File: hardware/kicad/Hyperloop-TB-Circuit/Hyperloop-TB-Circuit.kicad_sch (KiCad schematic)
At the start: 12 parts, among them J1 Conn_01x02, J2 Conn_01x02, Q1 IRLZ44N

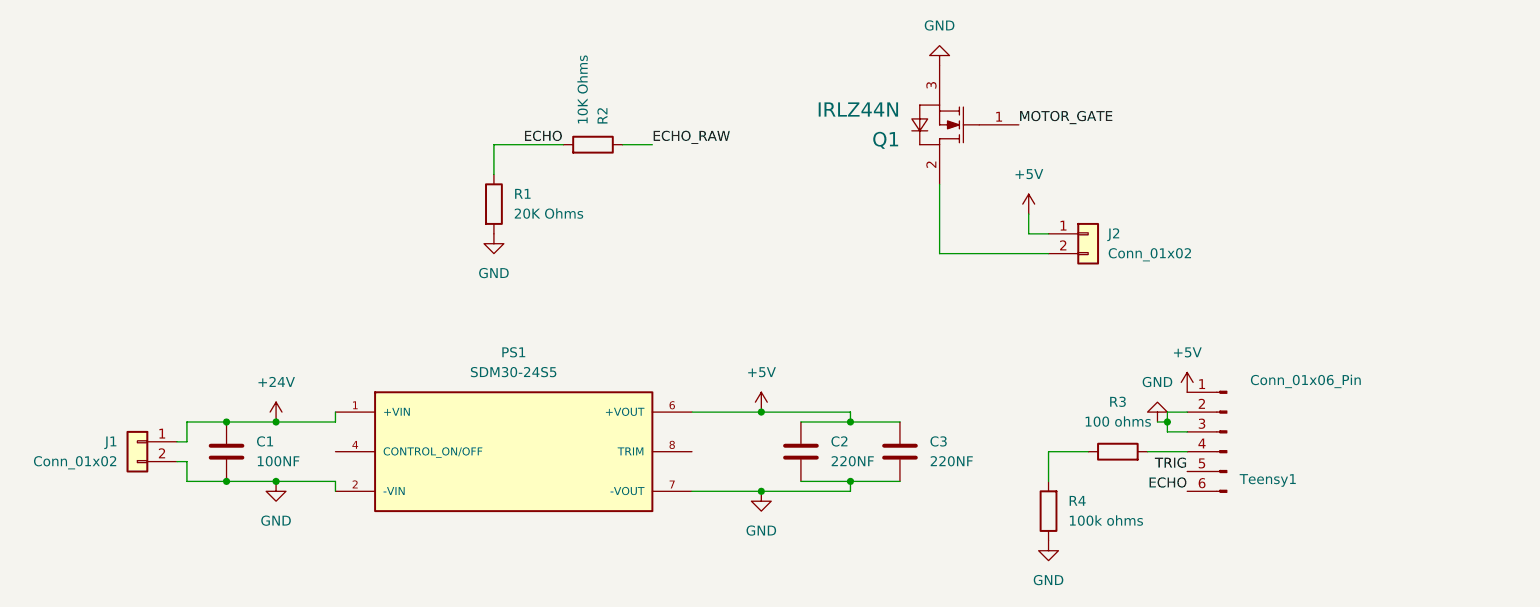
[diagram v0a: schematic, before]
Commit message: updated schematic and pcb
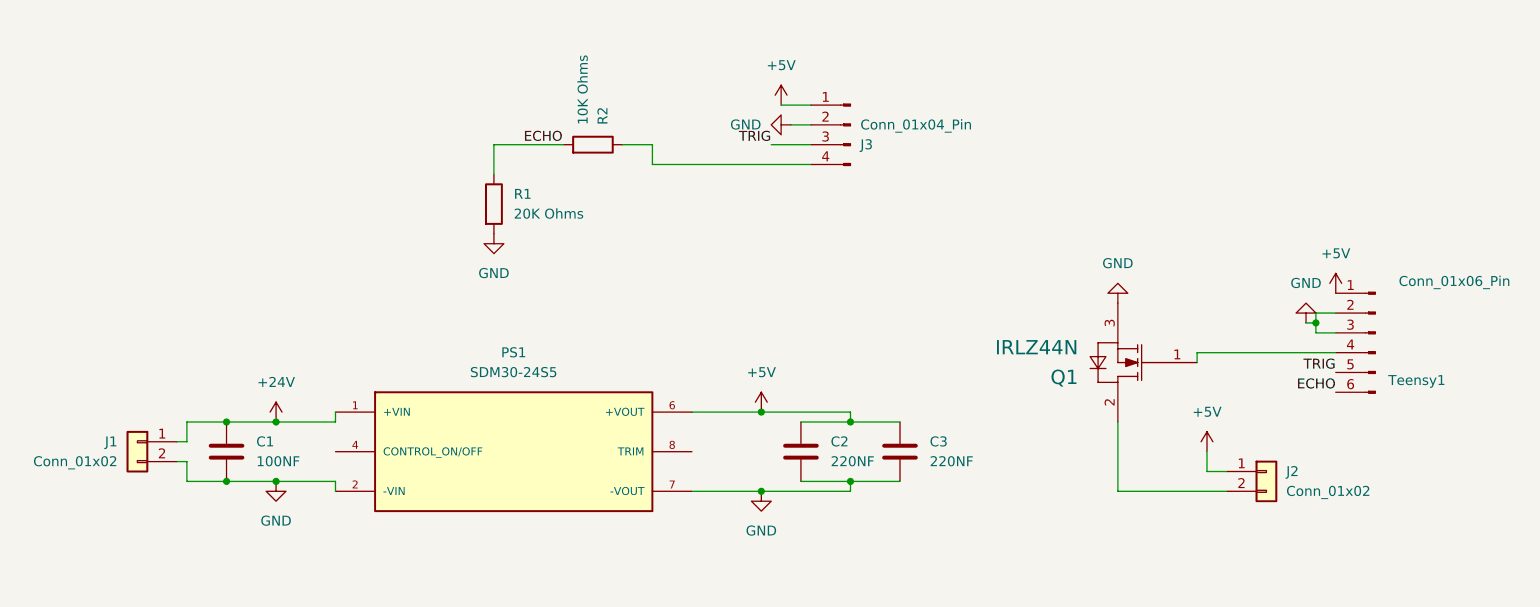
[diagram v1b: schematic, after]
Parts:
- removed R3: 100 ohms, Resistor_THT:R_Axial_DIN0204_L3.6mm_D1.6mm_P7.62mm_Horizontal, symbol Device:R
- removed R4: 100k ohms, Resistor_THT:R_Axial_DIN0204_L3.6mm_D1.6mm_P7.62mm_Horizontal, symbol Device:R
- added J3: Conn_01x04_Pin, Connector_Samtec_HPM_THT:Samtec_HPM-04-01-x-S_Straight_1x04_Pitch5.08mm, symbol Connector:Conn_01x04_Pin
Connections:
- net MOTOR_GATE is gone; now on an unnamed net: Q1.1 (GATE)
- net +5V: now also J3.1 (Pin_1)
- net GND: now also J3.2 (Pin_2)
- net TRIG: now also J3.3 (Pin_3)
- net ECHO_RAW: no longer names the net of R2.1
- net ECHO_RAW: now also J3.4 (Pin_4)
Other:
- moved on the sheet: J2, Q1, Teensy1
